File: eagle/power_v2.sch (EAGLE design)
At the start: 14 parts, among them X1 736880-49, X2 736880-49, X3 736880-49, X4 736880-49, X5 736880-49

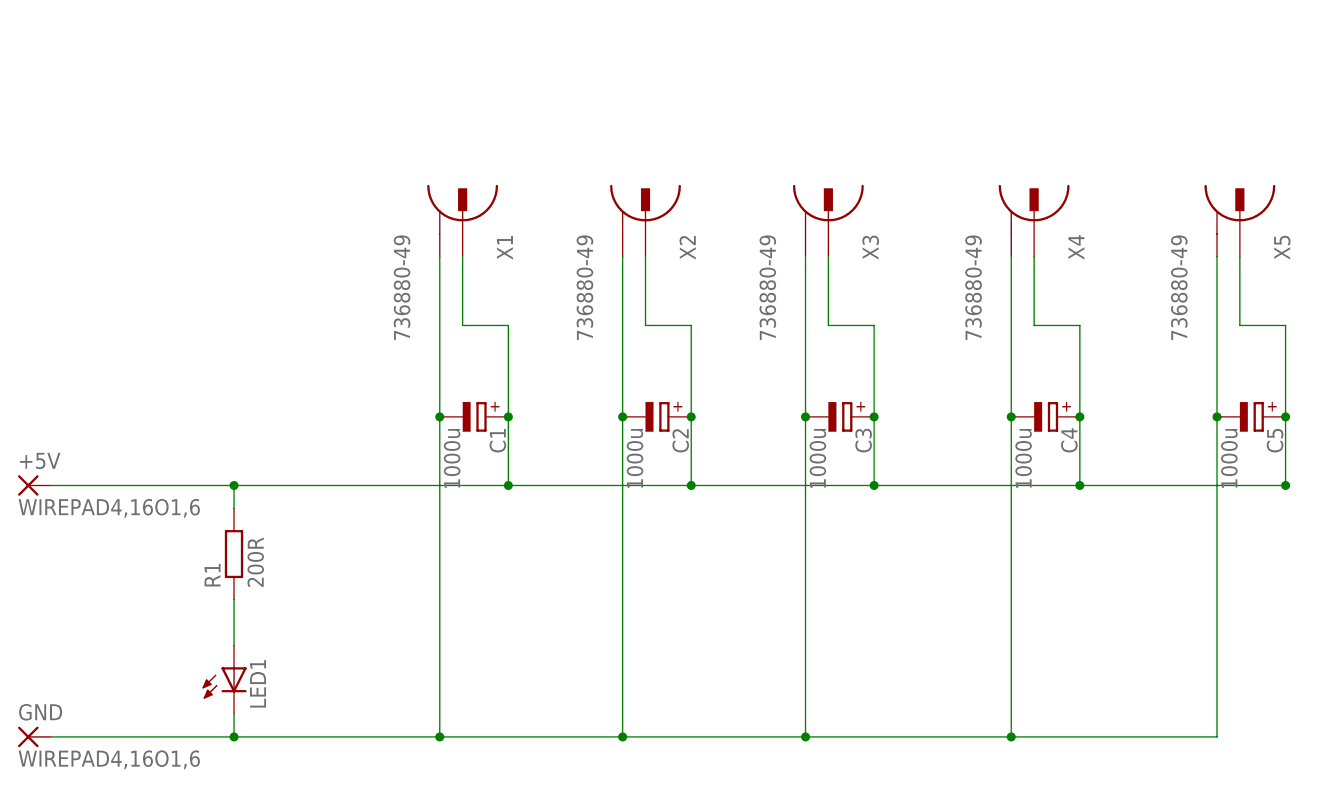
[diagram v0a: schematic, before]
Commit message: cinch -> svorkovnice
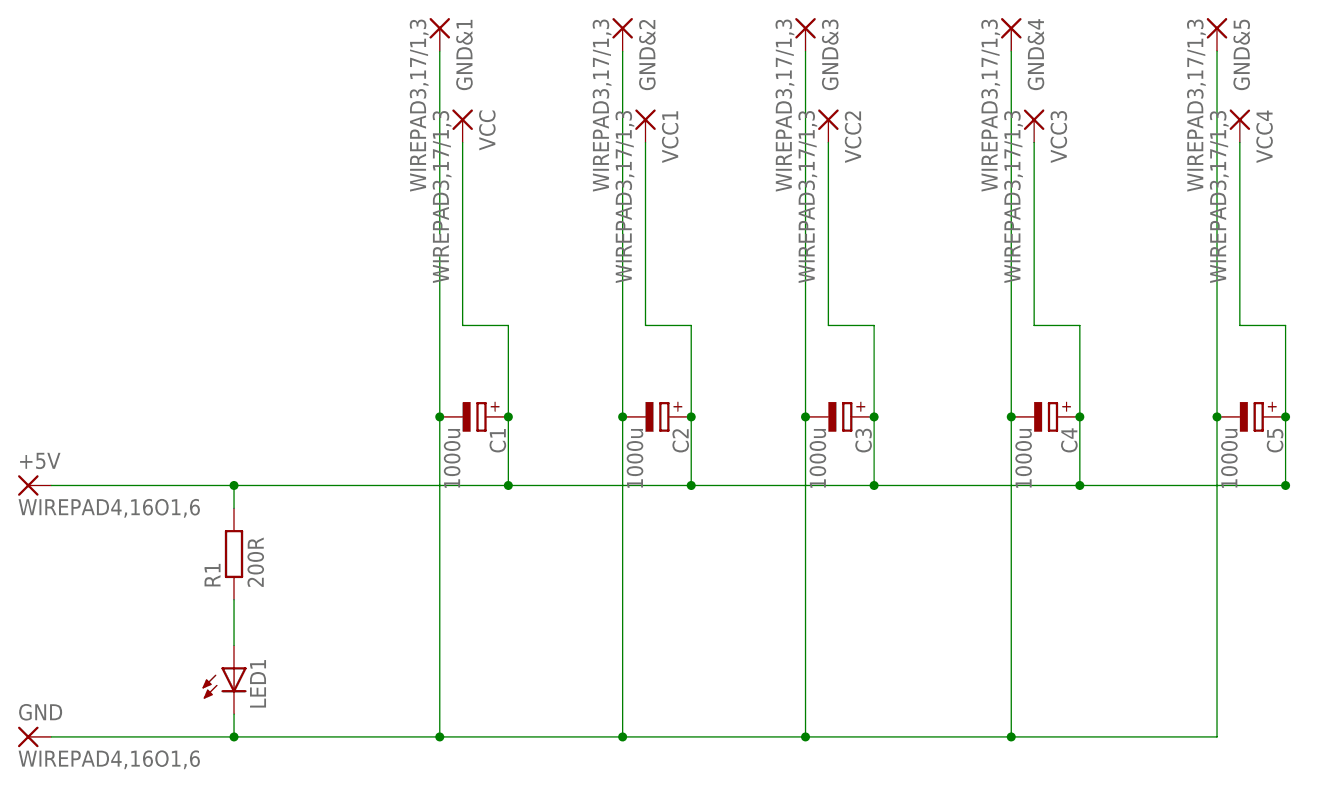
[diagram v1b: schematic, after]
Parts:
- removed X1, X2, X3, X4, X5: 736880-49, con-conrad:736880-49
- added GND&1, GND&2, GND&3, GND&4, GND&5, VCC, VCC1, VCC2, VCC3, VCC4: WIREPAD3,17/1,3, wirepad:WIREPAD3,17/1,3
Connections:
- new net N$1: GND&1.P
- net GND: now also GND&2.P, GND&3.P, GND&4.P, GND&5.P; no longer X1.2, X2.2, X3.2, X4.2, X5.2
- net N$6: now also VCC.P, VCC1.P, VCC2.P, VCC3.P, VCC4.P; no longer X1.1, X2.1, X3.1, X4.1, X5.1
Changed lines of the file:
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@@
 <setting verticaltext="up"/>
 </settings>
-<grid distance="0.1" unitdist="inch" unit="inch" style="lines" multiple="1" display="yes" altdistance="0.01" altunitdist="inch" altunit="inch"/>
+<grid distance="0.1" unitdist="inch" unit="inch" style="lines" multiple="1" display="no" altdistance="0.01" altunitdist="inch" altunit="inch"/>
 <layers>
 <layer number="1" name="Top" color="4" fill="1" visible="no" active="no"/>
@@
 <part name="+5V" library="wirepad" deviceset="WIREPAD" device="4,16O1,6"/>
 <part name="GND" library="wirepad" deviceset="WIREPAD" device="4,16O1,6"/>
-<part name="X1" library="con-conrad" deviceset="736880-49" device=""/>
 <part name="LED1" library="led" deviceset="LED" device="5MM"/>
 <part name="R1" library="resistor" deviceset="R-EU_" device="R1206" value="200R"/>
 <part name="C1" library="resistor" deviceset="CPOL-EU" device="E5-10.5" value="1000u"/>
-<part name="X2" library="con-conrad" deviceset="736880-49" device=""/>
 <part name="C2" library="resistor" deviceset="CPOL-EU" device="E5-10.5" value="1000u"/>
-<part name="X3" library="con-conrad" deviceset="736880-49" device=""/>
 <part name="C3" library="resistor" deviceset="CPOL-EU" device="E5-10.5" value="1000u"/>
-<part name="X4" library="con-conrad" deviceset="736880-49" device=""/>
 <part name="C4" library="resistor" deviceset="CPOL-EU" device="E5-10.5" value="1000u"/>
-<part name="X5" library="con-conrad" deviceset="736880-49" device=""/>
 <part name="C5" library="resistor" deviceset="CPOL-EU" device="E5-10.5" value="1000u"/>
+<part name="GND&amp;1" library="wirepad" deviceset="WIREPAD" device="3,17/1,3"/>
+<part name="VCC" library="wirepad" deviceset="WIREPAD" device="3,17/1,3"/>
+<part name="GND&amp;2" library="wirepad" deviceset="WIREPAD" device="3,17/1,3"/>
+<part name="VCC1" library="wirepad" deviceset="WIREPAD" device="3,17/1,3"/>
+<part name="GND&amp;3" library="wirepad" deviceset="WIREPAD" device="3,17/1,3"/>
+<part name="VCC2" library="wirepad" deviceset="WIREPAD" device="3,17/1,3"/>
+<part name="GND&amp;4" library="wirepad" deviceset="WIREPAD" device="3,17/1,3"/>
+<part name="VCC3" library="wirepad" deviceset="WIREPAD" device="3,17/1,3"/>
+<part name="GND&amp;5" library="wirepad" deviceset="WIREPAD" device="3,17/1,3"/>
+<part name="VCC4" library="wirepad" deviceset="WIREPAD" device="3,17/1,3"/>
 </parts>
 <sheets>
@@
 <instance part="+5V" gate="G$1" x="0" y="63.5"/>
 <instance part="GND" gate="G$1" x="0" y="35.56"/>
-<instance part="X1" gate="G$1" x="48.26" y="91.44" rot="R270"/>
 <instance part="LED1" gate="G$1" x="22.86" y="43.18"/>
 <instance part="R1" gate="G$1" x="22.86" y="55.88" rot="R90"/>
 <instance part="C1" gate="G$1" x="50.8" y="71.12" rot="R270"/>
-<instance part="X2" gate="G$1" x="68.58" y="91.44" rot="R270"/>
 <instance part="C2" gate="G$1" x="71.12" y="71.12" rot="R270"/>
-<instance part="X3" gate="G$1" x="88.9" y="91.44" rot="R270"/>
 <instance part="C3" gate="G$1" x="91.44" y="71.12" rot="R270"/>
-<instance part="X4" gate="G$1" x="111.76" y="91.44" rot="R270"/>
 <instance part="C4" gate="G$1" x="114.3" y="71.12" rot="R270"/>
-<instance part="X5" gate="G$1" x="134.62" y="91.44" rot="R270"/>
 <instance part="C5" gate="G$1" x="137.16" y="71.12" rot="R270"/>
+<instance part="GND&amp;1" gate="G$1" x="45.72" y="114.3" rot="R270"/>
+<instance part="VCC" gate="G$1" x="48.26" y="104.14" rot="R270"/>
+<instance part="GND&amp;2" gate="G$1" x="66.04" y="114.3" rot="R270"/>
+<instance part="VCC1" gate="G$1" x="68.58" y="104.14" rot="R270"/>
+<instance part="GND&amp;3" gate="G$1" x="86.36" y="114.3" rot="R270"/>
+<instance part="VCC2" gate="G$1" x="88.9" y="104.14" rot="R270"/>
+<instance part="GND&amp;4" gate="G$1" x="109.22" y="114.3" rot="R270"/>
+<instance part="VCC3" gate="G$1" x="111.76" y="104.14" rot="R270"/>
+<instance part="GND&amp;5" gate="G$1" x="132.08" y="114.3" rot="R270"/>
+<instance part="VCC4" gate="G$1" x="134.62" y="104.14" rot="R270"/>
 </instances>
 <busses>
@@
 <net name="GND" class="0">
 <segment>
-<pinref part="X1" gate="G$1" pin="2"/>
 <pinref part="C1" gate="G$1" pin="-"/>
 <wire x1="45.72" y1="88.9" x2="45.72" y2="71.12" width="0.1524" layer="91"/>
 <junction x="45.72" y="71.12"/>
-<pinref part="X2" gate="G$1" pin="2"/>
 <pinref part="C2" gate="G$1" pin="-"/>
-<wire x1="66.04" y1="88.9" x2="66.04" y2="71.12" width="0.1524" layer="91"/>
 <junction x="66.04" y="71.12"/>
-<pinref part="X3" gate="G$1" pin="2"/>
 <pinref part="C3" gate="G$1" pin="-"/>
-<wire x1="86.36" y1="88.9" x2="86.36" y2="71.12" width="0.1524" layer="91"/>
 <junction x="86.36" y="71.12"/>
-<pinref part="X4" gate="G$1" pin="2"/>
 <pinref part="C4" gate="G$1" pin="-"/>
-<wire x1="109.22" y1="88.9" x2="109.22" y2="71.12" width="0.1524" layer="91"/>
 <junction x="109.22" y="71.12"/>
-<pinref part="X5" gate="G$1" pin="2"/>
 <pinref part="C5" gate="G$1" pin="-"/>
-<wire x1="132.08" y1="88.9" x2="132.08" y2="71.12" width="0.1524" layer="91"/>
 <junction x="132.08" y="71.12"/>
 <pinref part="GND" gate="G$1" pin="P"/>
@@
 <wire x1="22.86" y1="38.1" x2="22.86" y2="35.56" width="0.1524" layer="91"/>
 <junction x="22.86" y="35.56"/>
+<pinref part="GND&amp;2" gate="G$1" pin="P"/>
+<wire x1="66.04" y1="71.12" x2="66.04" y2="111.76" width="0.1524" layer="91"/>
+<pinref part="GND&amp;3" gate="G$1" pin="P"/>
+<wire x1="86.36" y1="71.12" x2="86.36" y2="111.76" width="0.1524" layer="91"/>
+<pinref part="GND&amp;4" gate="G$1" pin="P"/>
+<wire x1="109.22" y1="71.12" x2="109.22" y2="111.76" width="0.1524" layer="91"/>
+<pinref part="GND&amp;5" gate="G$1" pin="P"/>
+<wire x1="132.08" y1="71.12" x2="132.08" y2="111.76" width="0.1524" layer="91"/>
 </segment>
 </net>
@@
 <wire x1="93.98" y1="71.12" x2="93.98" y2="81.28" width="0.1524" layer="91"/>
 <wire x1="93.98" y1="81.28" x2="88.9" y2="81.28" width="0.1524" layer="91"/>
-<pinref part="X3" gate="G$1" pin="1"/>
-<wire x1="88.9" y1="81.28" x2="88.9" y2="88.9" width="0.1524" layer="91"/>
 <junction x="93.98" y="71.12"/>
 <pinref part="C4" gate="G$1" pin="+"/>
 <wire x1="116.84" y1="71.12" x2="116.84" y2="81.28" width="0.1524" layer="91"/>
 <wire x1="116.84" y1="81.28" x2="111.76" y2="81.28" width="0.1524" layer="91"/>
-<pinref part="X4" gate="G$1" pin="1"/>
-<wire x1="111.76" y1="81.28" x2="111.76" y2="88.9" width="0.1524" layer="91"/>
 <junction x="116.84" y="71.12"/>
 <pinref part="C1" gate="G$1" pin="+"/>
 <wire x1="53.34" y1="71.12" x2="53.34" y2="81.28" width="0.1524" layer="91"/>
 <wire x1="53.34" y1="81.28" x2="48.26" y2="81.28" width="0.1524" layer="91"/>
-<pinref part="X1" gate="G$1" pin="1"/>
-<wire x1="48.26" y1="81.28" x2="48.26" y2="88.9" width="0.1524" layer="91"/>
 <junction x="53.34" y="71.12"/>
 <pinref part="+5V" gate="G$1" pin="P"/>
@@
 <wire x1="73.66" y1="71.12" x2="73.66" y2="81.28" width="0.1524" layer="91"/>
 <wire x1="73.66" y1="81.28" x2="68.58" y2="81.28" width="0.1524" layer="91"/>
-<pinref part="X2" gate="G$1" pin="1"/>
-<wire x1="68.58" y1="81.28" x2="68.58" y2="88.9" width="0.1524" layer="91"/>
 <junction x="73.66" y="71.12"/>
 <wire x1="53.34" y1="63.5" x2="73.66" y2="63.5" width="0.1524" layer="91"/>
@@
 <wire x1="139.7" y1="71.12" x2="139.7" y2="81.28" width="0.1524" layer="91"/>
 <wire x1="139.7" y1="81.28" x2="134.62" y2="81.28" width="0.1524" layer="91"/>
-<pinref part="X5" gate="G$1" pin="1"/>
-<wire x1="134.62" y1="81.28" x2="134.62" y2="88.9" width="0.1524" layer="91"/>
 <junction x="139.7" y="71.12"/>
 <wire x1="73.66" y1="63.5" x2="93.98" y2="63.5" width="0.1524" layer="91"/>
@@
 <wire x1="22.86" y1="60.96" x2="22.86" y2="63.5" width="0.1524" layer="91"/>
 <junction x="22.86" y="63.5"/>
+<pinref part="VCC" gate="G$1" pin="P"/>
+<wire x1="48.26" y1="101.6" x2="48.26" y2="81.28" width="0.1524" layer="91"/>
+<pinref part="VCC1" gate="G$1" pin="P"/>
+<wire x1="68.58" y1="81.28" x2="68.58" y2="101.6" width="0.1524" layer="91"/>
+<pinref part="VCC2" gate="G$1" pin="P"/>
+<wire x1="88.9" y1="81.28" x2="88.9" y2="101.6" width="0.1524" layer="91"/>
+<pinref part="VCC3" gate="G$1" pin="P"/>
+<wire x1="111.76" y1="81.28" x2="111.76" y2="101.6" width="0.1524" layer="91"/>
+<pinref part="VCC4" gate="G$1" pin="P"/>
+<wire x1="134.62" y1="81.28" x2="134.62" y2="101.6" width="0.1524" layer="91"/>
 </segment>
 </net>
@@
 </segment>
 </net>
+<net name="N$1" class="0">
+<segment>
+<pinref part="GND&amp;1" gate="G$1" pin="P"/>
+<wire x1="45.72" y1="91.44" x2="45.72" y2="111.76" width="0.1524" layer="91"/>
+</segment>
+</net>
